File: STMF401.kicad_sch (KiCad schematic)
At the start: 26 parts, among them J6 Conn_01x04_Pin, U3 STM32F407VETx, Y1 X322525MQB4SI, Y2 SMD03215C2

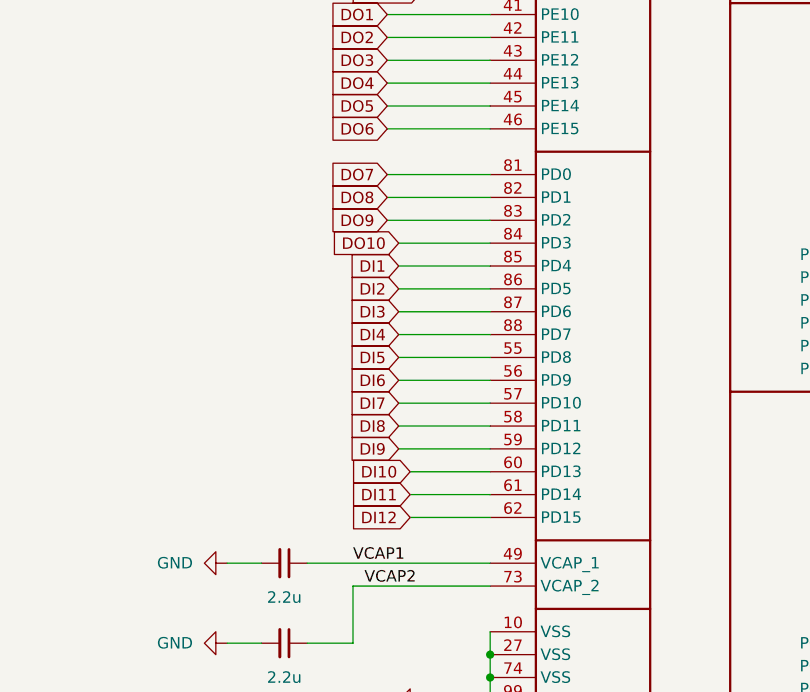
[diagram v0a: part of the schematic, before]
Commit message: feat: разведены линии DI большая часть
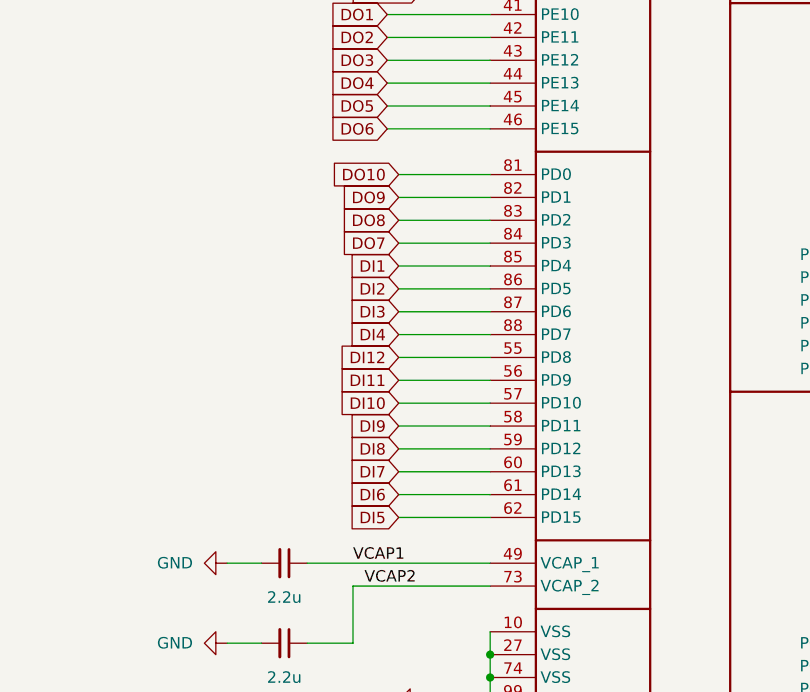
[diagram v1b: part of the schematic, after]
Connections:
- net DI10: now also U3.57 (PD10); no longer U3.60 (PD13)
- net DI11: now also U3.56 (PD9); no longer U3.61 (PD14)
- net DI12: now also U3.55 (PD8); no longer U3.62 (PD15)
- net DI5: now also U3.62 (PD15); no longer U3.55 (PD8)
- net DI6: now also U3.61 (PD14); no longer U3.56 (PD9)
- net DI7: now also U3.60 (PD13); no longer U3.57 (PD10)
- net DI8: now also U3.59 (PD12); no longer U3.58 (PD11)
- net DI9: now also U3.58 (PD11); no longer U3.59 (PD12)
- net DO10: now also U3.81 (PD0); no longer U3.84 (PD3)
- net DO7: now also U3.84 (PD3); no longer U3.81 (PD0)
- net DO8: now also U3.83 (PD2); no longer U3.82 (PD1)
- net DO9: now also U3.82 (PD1); no longer U3.83 (PD2)
